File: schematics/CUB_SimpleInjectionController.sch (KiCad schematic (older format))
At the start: 19 parts, among them P1 CONN_POWER, P2 CONN_01X03, Q1 IRF3710, U1 Arduino_NANO

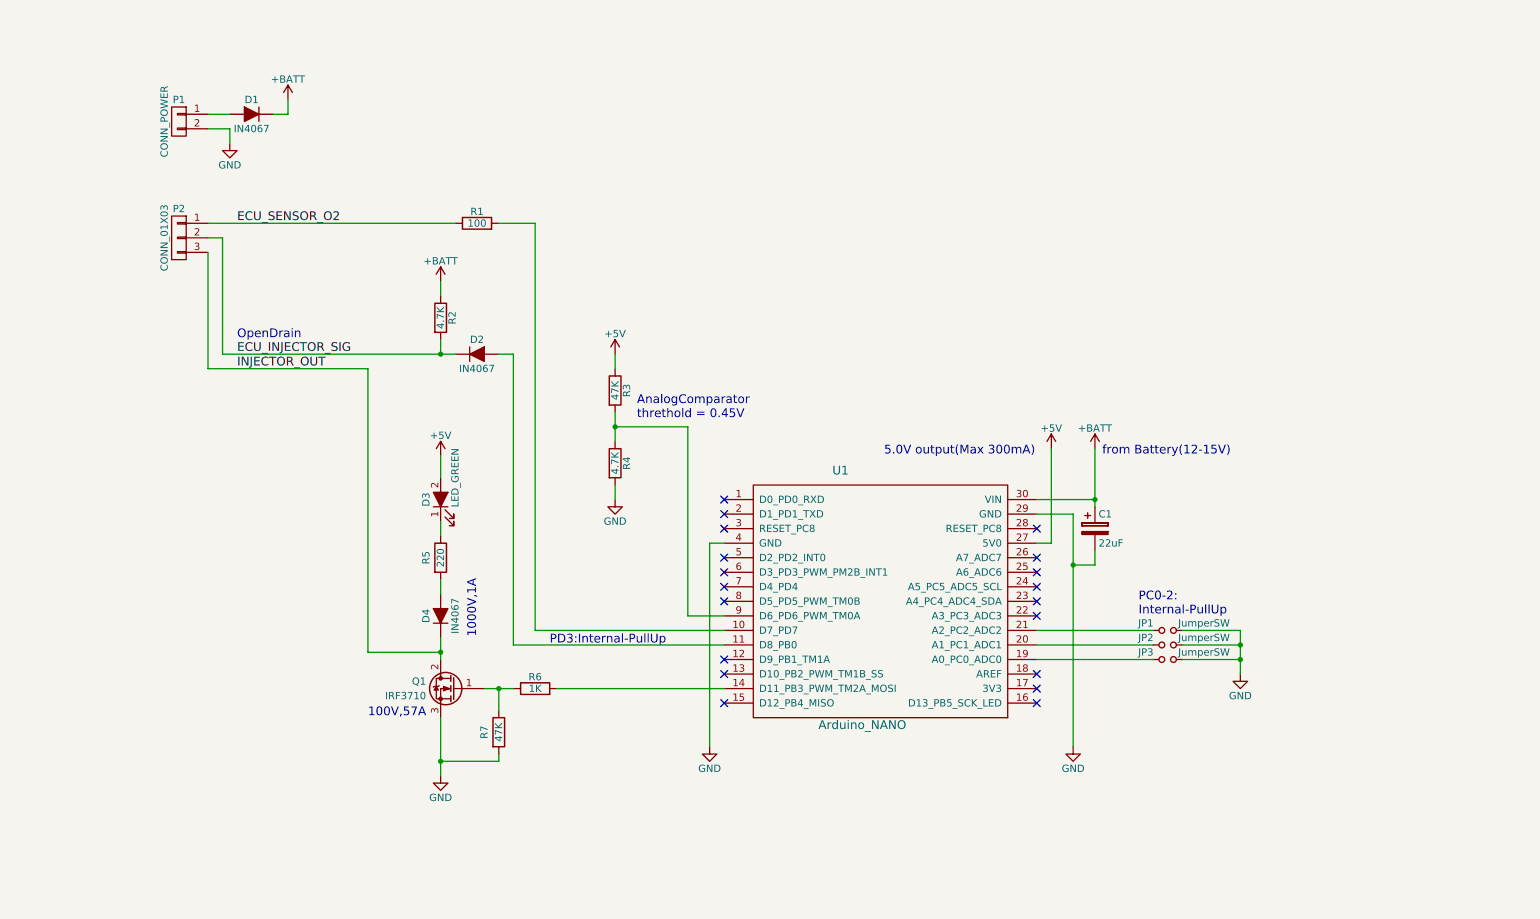
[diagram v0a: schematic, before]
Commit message: Update sketch and schematics. It's alpha version.
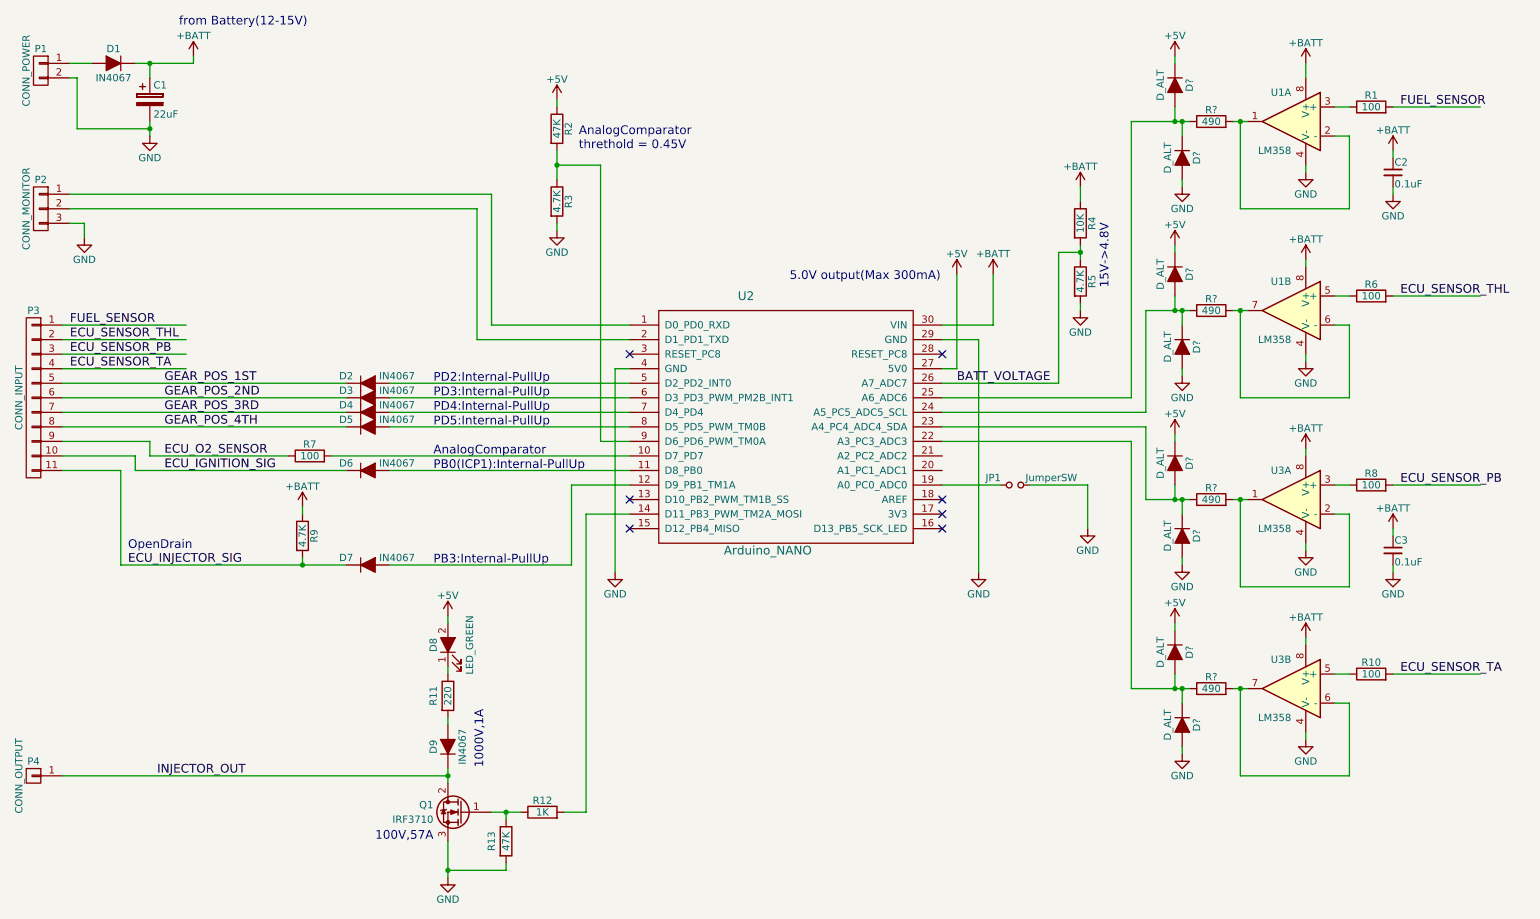
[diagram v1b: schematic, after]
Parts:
- removed JP2, JP3: JumperSW, symbol Jumper_NO_Small
- added C2, C3: 0.1uF, symbol C_Small
- added D2, D3, D4, D5, D6: IN4067, symbol D_ALT
- added D? (x8): D_ALT, symbol D_ALT
- added P3: CONN_INPUT, symbol CONN_01X11
- added P4: CONN_OUTPUT, symbol CONN_01X01
- added R10, R6, R7, R8: 100, symbol R
- added R2: 47K, symbol R
- added R5: 4.7K, symbol R
- added R? (x4): 490, symbol R
- added U1, U3: LM358, symbol LM358
- P2: value CONN_01X03 -> CONN_MONITOR
- R3: value 47K -> 4.7K
- R4: value 4.7K -> 10K
- renumbered D2 to D7, D3 to D8, D4 to D9, R5 to R11, R6 to R12, R7 to R13, R2 to R9, U1 to U2
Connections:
- net labels added: BATT_VOLTAGE, ECU_IGNITION_SIG, ECU_O2_SENSOR, ECU_SENSOR_PB, ECU_SENSOR_TA, ECU_SENSOR_THL, FUEL_SENSOR, GEAR_POS_1ST, GEAR_POS_2ND, GEAR_POS_3RD, GEAR_POS_4TH
- net labels removed: ECU_SENSOR_O2
- wire segments 54 -> 148
- no-connect marks 19 -> 7
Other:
- note added: "15V->4.8V"
- note added: "AnalogComparator"
- note added: "PB0(ICP1):Internal-PullUp"
- note added: "PB3:Internal-PullUp"
- note added: "PD2:Internal-PullUp"
- note added: "PD4:Internal-PullUp"
- note added: "PD5:Internal-PullUp"
- note removed: "PC0-2:\nInternal-PullUp"
- moved on the sheet: C1, D1, D7, D8, D9, JP1, P1, Q1, R11, R12, R13, R9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
